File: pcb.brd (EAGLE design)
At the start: 121 x 83 mm, 22 parts

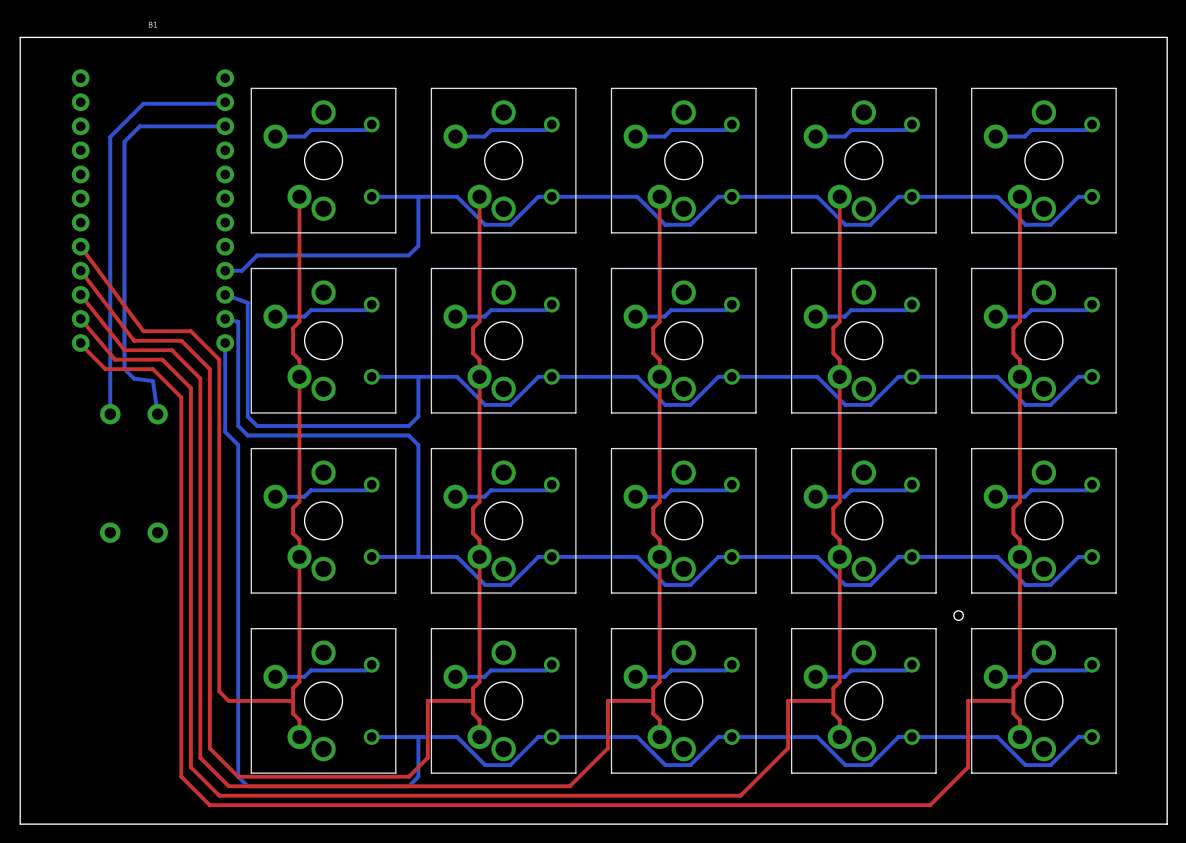
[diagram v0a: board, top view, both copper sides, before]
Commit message: Final design; ordered
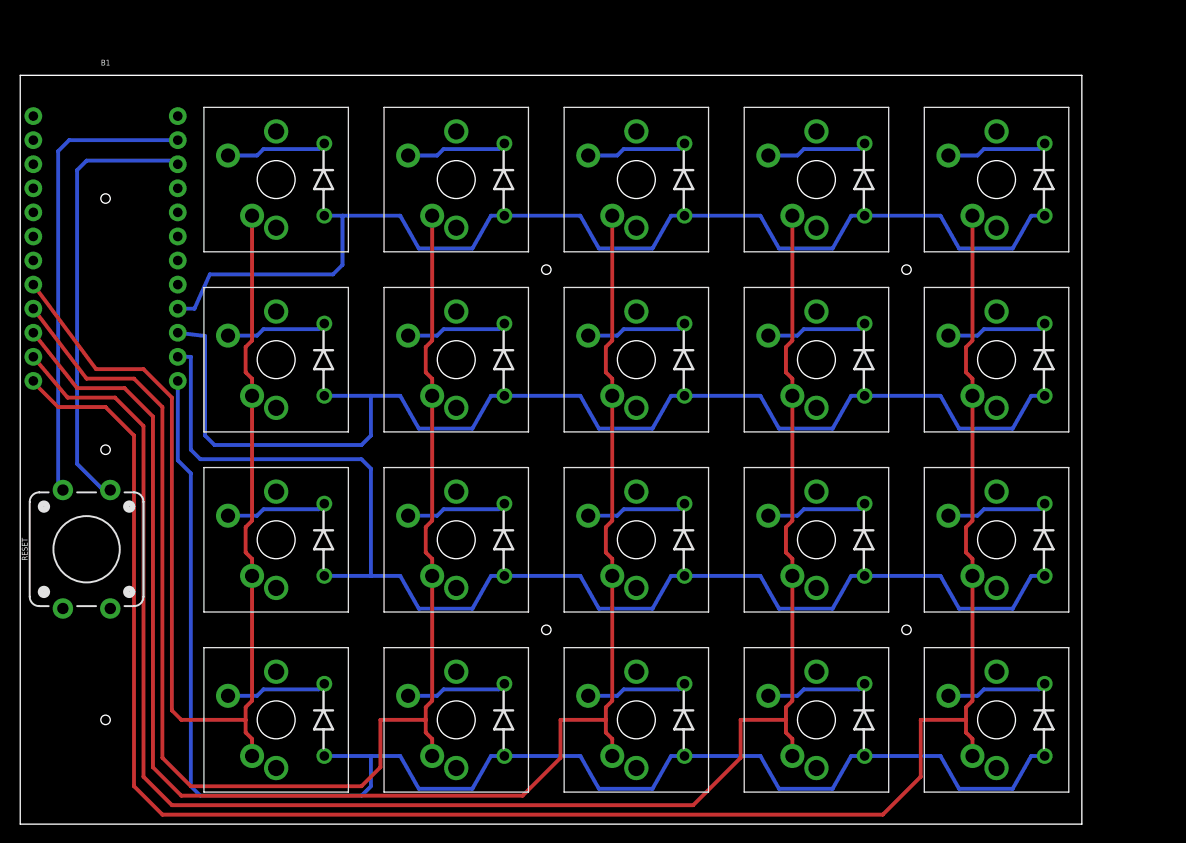
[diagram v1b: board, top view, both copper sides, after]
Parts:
- removed S1: RESET, SparkFun-Switches:TACTILE_SWITCH_PTH_12MM
- added RESET: RESET, SparkFun-Switches:TACTILE_SWITCH_PTH_12MM
- moved B1 6.40 mm to (9.00, 62.0)
- moved U$1 5.39 mm to (27.0, 68.0)
- moved U$10 5.39 mm to (103.0, 49.0)
- moved U$11 5.39 mm to (27.0, 30.0)
- moved U$12 5.39 mm to (46.0, 30.0)
- moved U$13 5.39 mm to (65.0, 30.0)
- moved U$14 5.39 mm to (84.0, 30.0)
- moved U$15 5.39 mm to (103.0, 30.0)
- moved U$16 5.39 mm to (27.0, 11.0)
- moved U$17 5.39 mm to (46.0, 11.0)
- moved U$18 5.39 mm to (65.0, 11.0)
- moved U$19 5.39 mm to (84.0, 11.0)
- moved U$2 5.39 mm to (46.0, 68.0)
- moved U$20 5.39 mm to (103.0, 11.0)
- moved U$3 5.39 mm to (65.0, 68.0)
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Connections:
- removed net N$28: B1.22, S1.3
- new net N$3: B1.23, RESET.3
- new net S$1: U$14.SW1, U$19.SW1, U$4.SW1, U$9.SW1
- new net S$2: U$10.SW1, U$15.SW1, U$20.SW1, U$5.SW1
- new net S$3: U$1.SW1, U$11.SW1, U$16.SW1, U$6.SW1
- net N$1: no longer U$1.SW1, U$11.SW1, U$16.SW1, U$6.SW1
- net N$26: now also B1.22, RESET.1; no longer B1.23, S1.1
- net N$4: no longer U$14.SW1, U$19.SW1, U$4.SW1, U$9.SW1
- net N$5: no longer U$10.SW1, U$15.SW1, U$20.SW1, U$5.SW1
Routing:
- net N$5: track 209.5 -> 146.8 mm
- net N$4: track 189.6 -> 127.0 mm
- net N$1: track 122.2 -> 61.5 mm
- net S$3: track 0.00 -> 58.7 mm
- net S$2: track 0.00 -> 58.7 mm
- net S$1: track 0.00 -> 58.7 mm
- net N$3: track 0.00 -> 49.1 mm
- net N$28: track 42.3 -> 0.00 mm
- net N$36: track 112.5 -> 117.5 mm
- net N$31: track 123.4 -> 128.1 mm
- net N$32: track 129.9 -> 134.5 mm
- net N$2: track 153.1 -> 149.1 mm
- net N$29: track 171.1 -> 167.1 mm
- net N$26: track 42.9 -> 46.8 mm
- net N$30: track 156.3 -> 158.6 mm
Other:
- board size 121 x 83 mm -> 112 x 79 mm
